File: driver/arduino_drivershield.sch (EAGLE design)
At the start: 21 parts, among them IC1 LB1973M, IC10 74HC14D, IC11 74HC14D, IC2 LB1973M, IC3 LB1973M, IC4 LB1973M, IC5 LB1973M, IC6 LB1973M, IC7 LB1973M, IC8 LB1973M, IC9 74HC14D, U1 ARDUINO_SHIELDLABEL

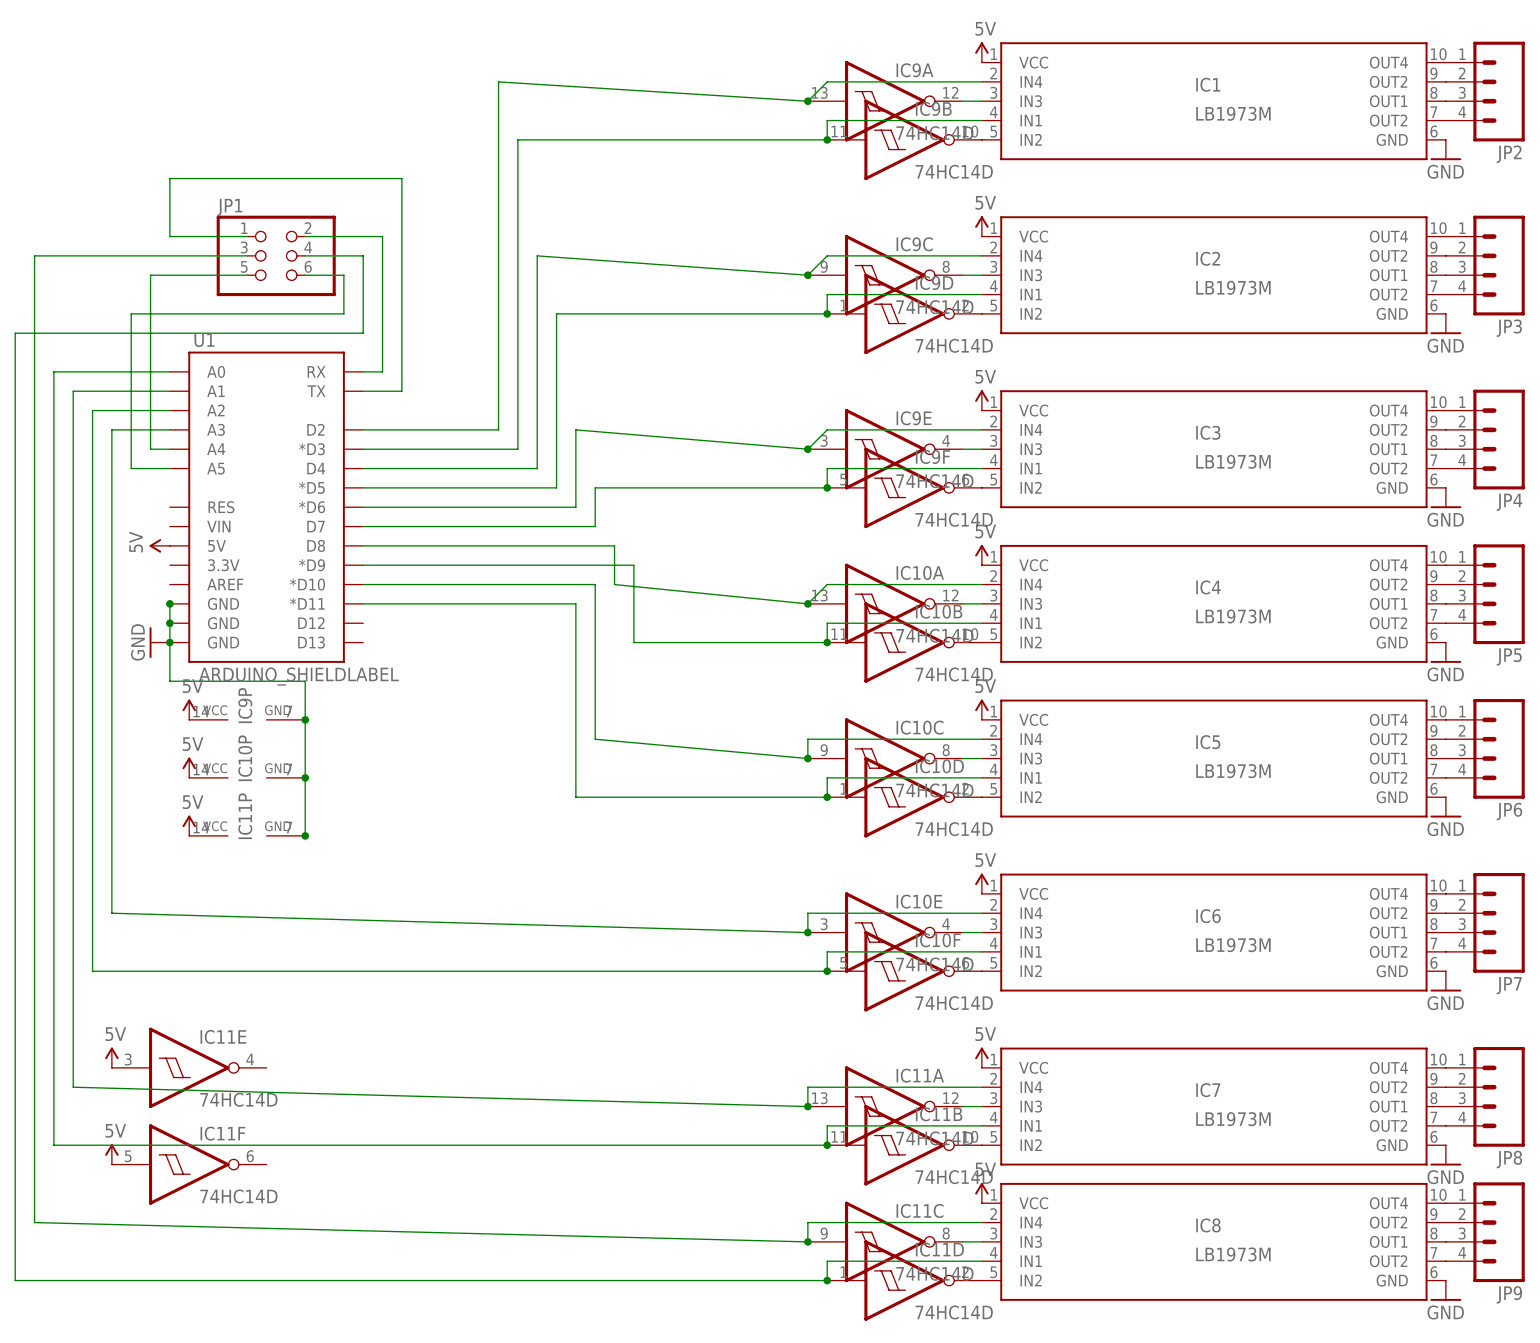
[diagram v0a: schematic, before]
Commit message: starting over...
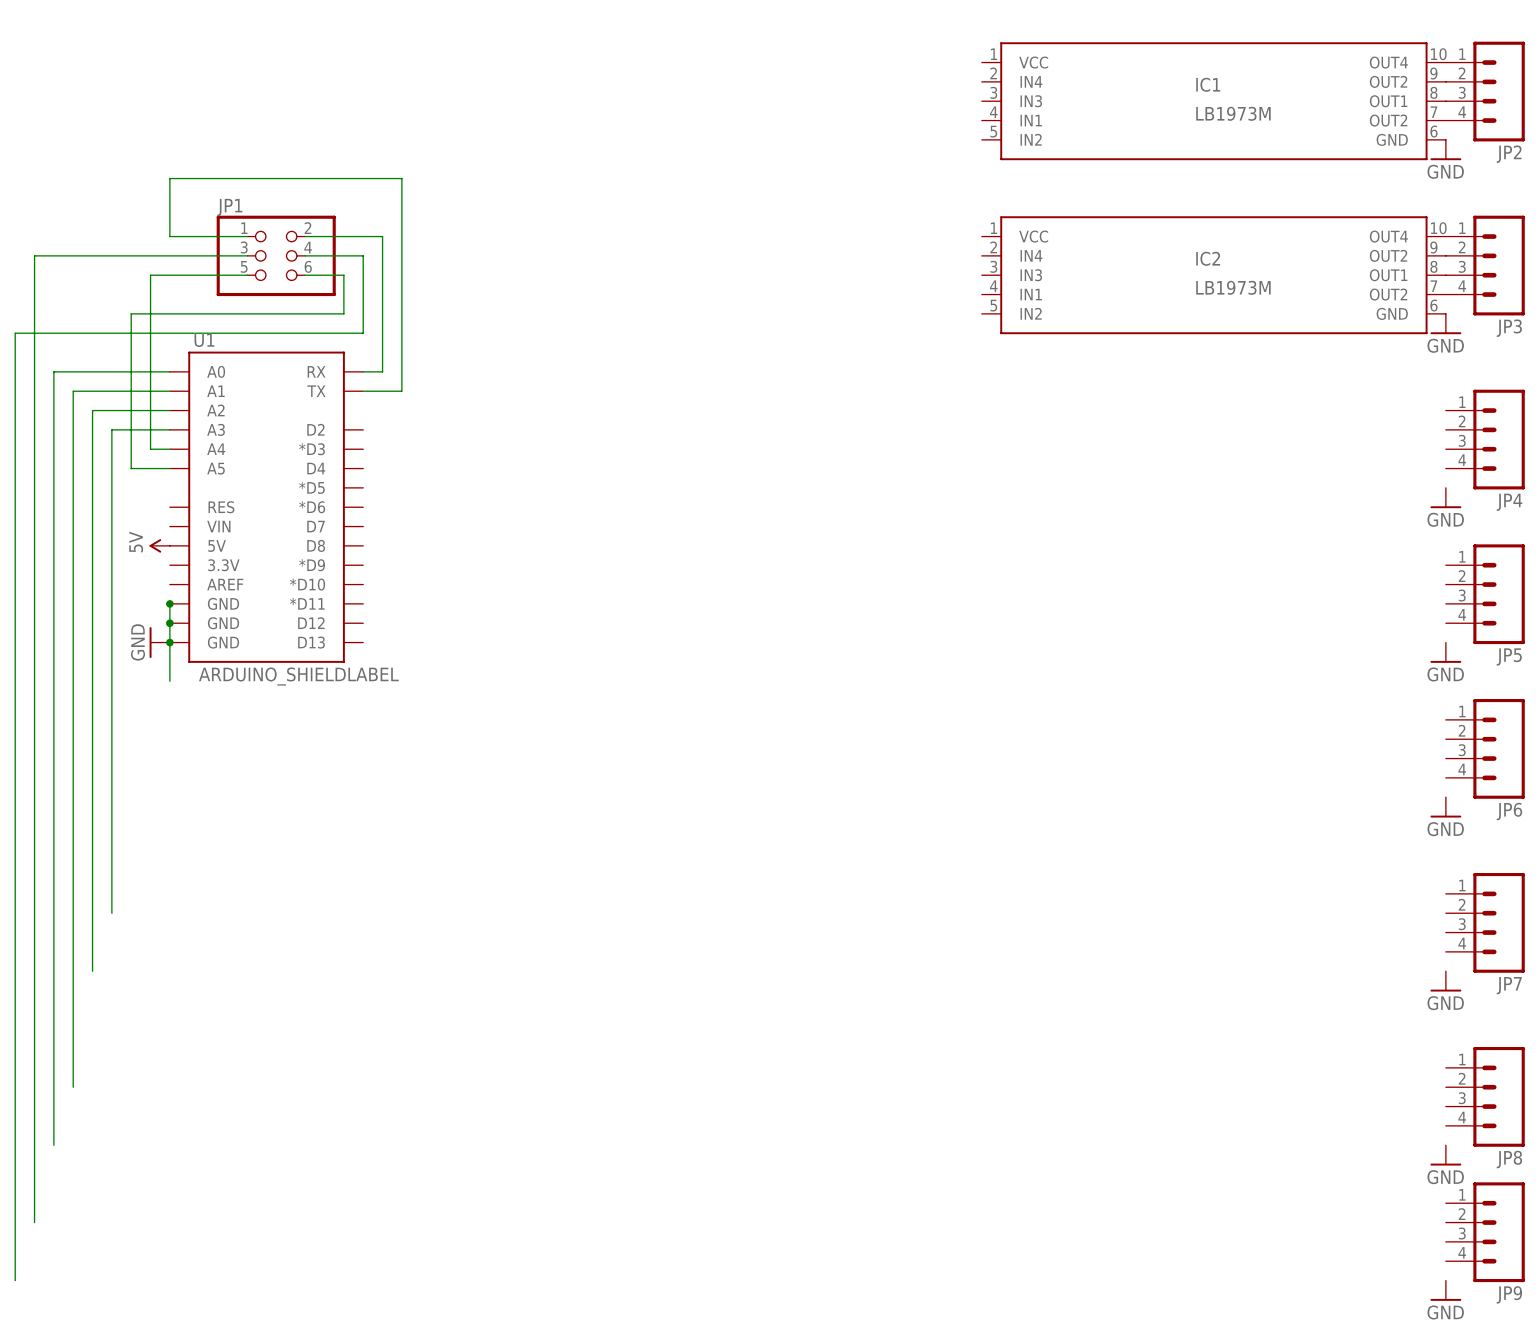
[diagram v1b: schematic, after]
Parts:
- removed IC10, IC11, IC9: 74HC14D, 74xx-eu:74HC14D
- removed IC3, IC4, IC5, IC6, IC7, IC8: LB1973M, LB1973M:LB1973M
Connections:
- removed net N$1 (its old number): IC2.IN3, IC9C.O
- removed net N$10: IC3.IN2, IC9F.O
- removed net N$15: IC3.IN3, IC9E.O
- removed net N$16: IC10B.O, IC4.IN2
- removed net N$17: IC1.IN4, IC9A.I, U1.D2
- removed net N$18: IC1.IN1, IC9B.I, U1.*D3
- removed net N$19: IC2.IN4, IC9C.I, U1.D4
- removed net N$2 (its old number): IC1.IN2, IC9B.O
- removed net N$20: IC2.IN1, IC9D.I, U1.*D5
- removed net N$21: IC3.IN4, IC9E.I, U1.*D6
- removed net N$22: IC3.IN1, IC9F.I, U1.D7
- removed net N$23: IC10A.I, IC4.IN4, U1.D8
- removed net N$24: IC10B.I, IC4.IN1, U1.*D9
- removed net N$25: IC10C.I, IC5.IN4, U1.*D10
- removed net N$26: IC10D.I, IC5.IN1, U1.*D11
- removed net N$33: IC10C.O, IC5.IN3
- removed net N$34: IC10D.O, IC5.IN2
- removed net N$35: IC3.OUT4, JP4.1
- removed net N$36: IC3.OUT2@1, JP4.2
- removed net N$37: IC3.OUT1, JP4.3
- removed net N$38: IC3.OUT2, JP4.4
- removed net N$39: IC10E.O, IC6.IN3
- removed net N$40: IC10F.O, IC6.IN2
- removed net N$41: IC11A.O, IC7.IN3
- removed net N$42: IC11B.O, IC7.IN2
- removed net N$43: IC4.OUT4, JP5.1
- removed net N$44: IC4.OUT2@1, JP5.2
- removed net N$45: IC4.OUT1, JP5.3
- removed net N$46: IC4.OUT2, JP5.4
- removed net N$47: IC11C.O, IC8.IN3
- removed net N$48: IC11D.O, IC8.IN2
- removed net N$49: IC5.OUT4, JP6.1
- removed net N$50: IC5.OUT2@1, JP6.2
- removed net N$51: IC5.OUT1, JP6.3
- removed net N$52: IC5.OUT2, JP6.4
- removed net N$53: IC6.OUT4, JP7.1
- removed net N$54: IC6.OUT2@1, JP7.2
- removed net N$55: IC6.OUT1, JP7.3
- removed net N$56: IC6.OUT2, JP7.4
- removed net N$57: IC7.OUT4, JP8.1
- removed net N$58: IC7.OUT2@1, JP8.2
- removed net N$59: IC7.OUT1, JP8.3
- removed net N$60: IC7.OUT2, JP8.4
- removed net N$61: IC8.OUT4, JP9.1
- removed net N$62: IC8.OUT2@1, JP9.2
- removed net N$63: IC8.OUT1, JP9.3
- removed net N$64: IC8.OUT2, JP9.4
- removed net N$7 (its old number): IC10A.O, IC4.IN3
- removed net N$8 (its old number): IC2.IN2, IC9D.O
- removed net N$9: IC1.IN3, IC9A.O
- net 5V: no longer IC1.VCC, IC10P.VCC, IC11E.I, IC11F.I, IC11P.VCC, IC2.VCC, IC3.VCC, IC4.VCC, IC5.VCC, IC6.VCC, IC7.VCC, IC8.VCC, IC9P.VCC
- net GND: no longer IC10P.GND, IC11P.GND, IC3.GND, IC4.GND, IC5.GND, IC6.GND, IC7.GND, IC8.GND, IC9P.GND
- net N$27: no longer IC10E.I, IC6.IN4
- net N$28: no longer IC10F.I, IC6.IN1
- net N$29: no longer IC11A.I, IC7.IN4
- net N$30: no longer IC11B.I, IC7.IN1
- net N$31: no longer IC11C.I, IC8.IN4
- net N$32: no longer IC11D.I, IC8.IN1
